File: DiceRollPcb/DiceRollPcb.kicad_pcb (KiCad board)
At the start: 2 copper layers, 96.5 x 68.6 mm, 20 parts, among them SW1 SW_Push, SW2 SW_Push, SW3 SW_Push, SW4 SW_Push, U1 RaspberryPiPico

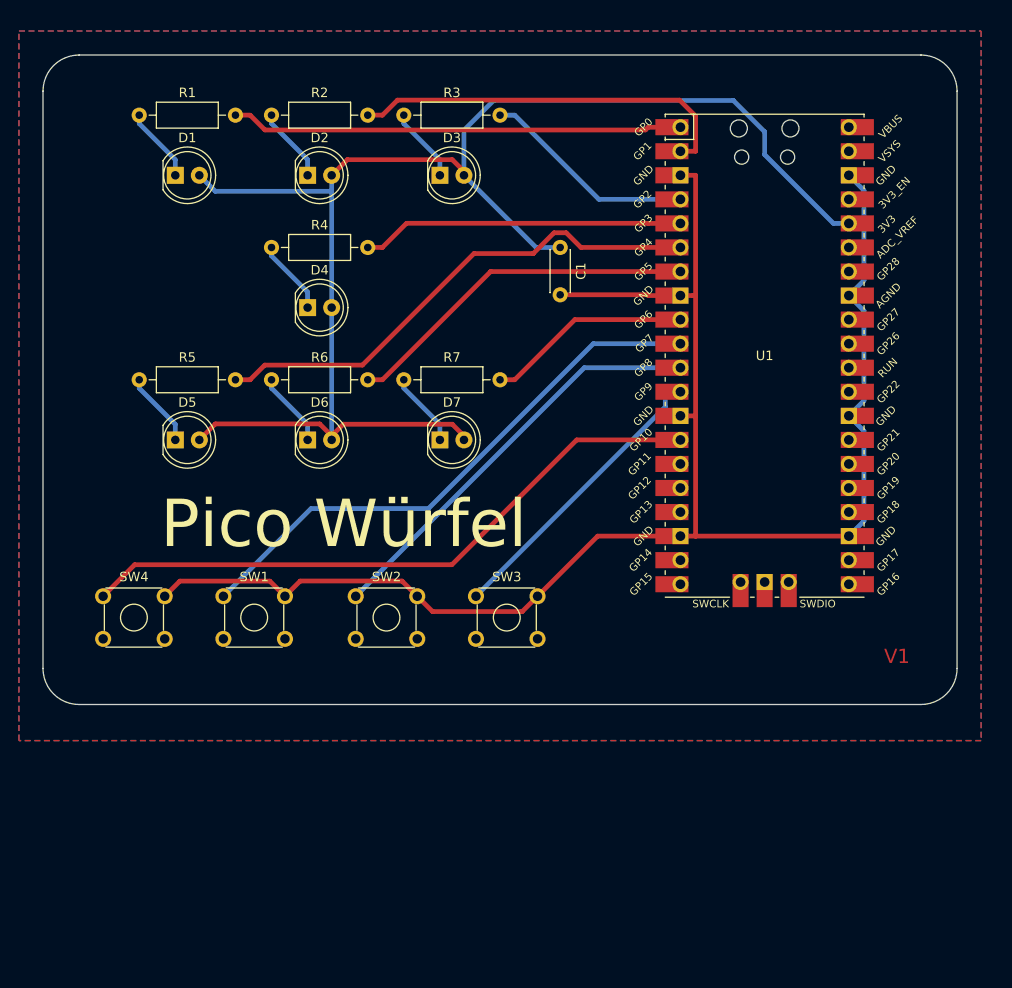
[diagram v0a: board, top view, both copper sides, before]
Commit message: Version 2
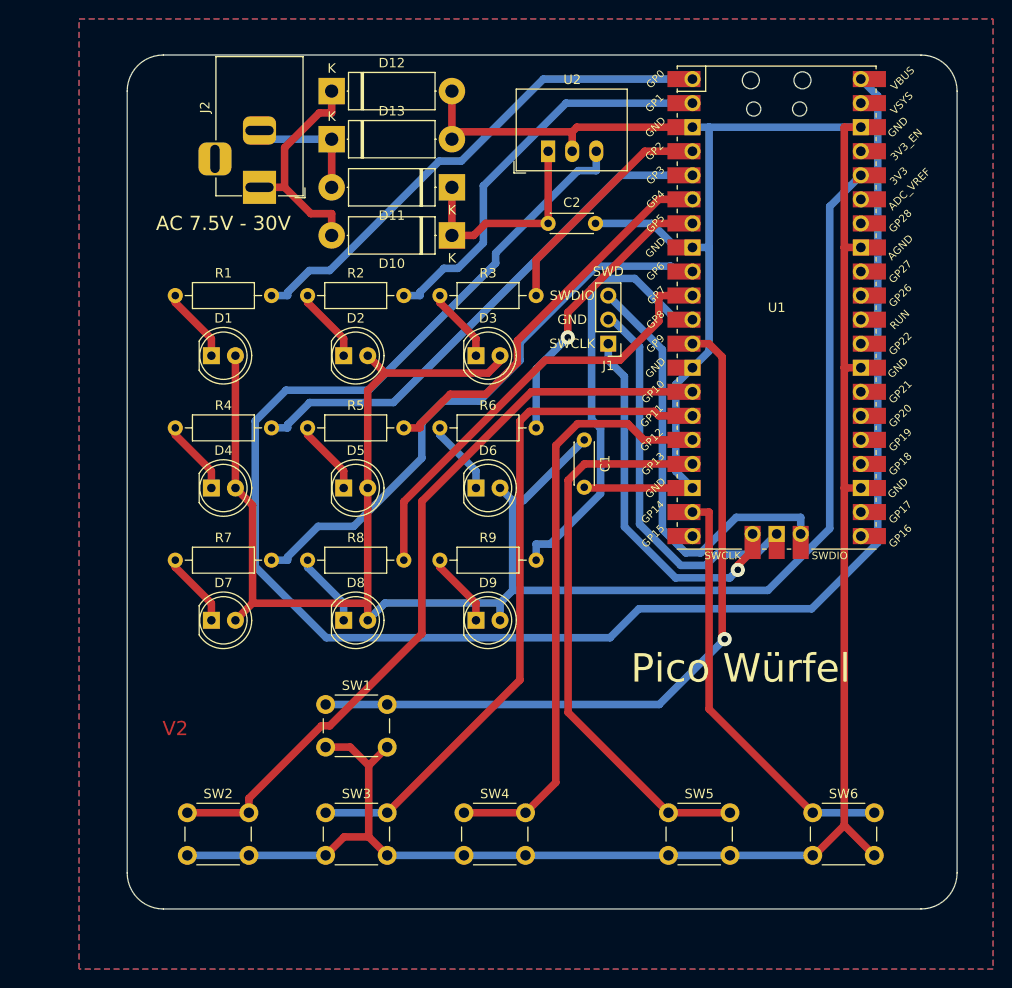
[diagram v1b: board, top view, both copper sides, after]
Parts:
- added C2: 4.7µF, Capacitor_THT:C_Disc_D4.3mm_W1.9mm_P5.00mm, F.Cu at (151.1, 74.9)
- added D10: D, Diode_THT:D_5W_P12.70mm_Horizontal, F.Cu at (141.0, 76.2)
- added D11: D, Diode_THT:D_5W_P12.70mm_Horizontal, F.Cu at (141.0, 71.1)
- added D12: D, Diode_THT:D_5W_P12.70mm_Horizontal, F.Cu at (128.3, 61.0)
- added D13: D, Diode_THT:D_5W_P12.70mm_Horizontal, F.Cu at (128.3, 66.0)
- added D8: LED, LED_THT:LED_D5.0mm, F.Cu at (129.5, 116.8)
- added D9: LED, LED_THT:LED_D5.0mm, F.Cu at (143.5, 116.8)
- added J1: Conn_01x03_Male, Connector_PinHeader_2.54mm:PinHeader_1x03_P2.54mm_Vertical, F.Cu at (157.5, 87.6)
- added J2: Barrel_Jack, Connector_BarrelJack:BarrelJack_Horizontal, F.Cu at (120.7, 71.1)
- added R8: R, Resistor_THT:R_Axial_DIN0207_L6.3mm_D2.5mm_P10.16mm_Horizontal, F.Cu at (125.7, 110.5)
- added R9: R, Resistor_THT:R_Axial_DIN0207_L6.3mm_D2.5mm_P10.16mm_Horizontal, F.Cu at (139.7, 110.5)
- added SW5: SW_Push, Button_Switch_THT:SW_PUSH_6mm, F.Cu at (163.8, 137.2)
- added SW6: SW_Push, Button_Switch_THT:SW_PUSH_6mm, F.Cu at (179.1, 137.2)
- added U2: R-785.0-0.5, Converter_DCDC:Converter_DCDC_RECOM_R-78E-0.5_THT, F.Cu at (151.1, 67.3)
- SW1, SW2, SW3, SW4: footprint Button_Switch_THT:SW_TH_Tactile_Omron_B3F-10xx -> Button_Switch_THT:SW_PUSH_6mm
- moved SW4 44.4 mm to (142.2, 137.2)
- moved D7 30.7 mm to (115.6, 116.8)
- moved R7 30.7 mm to (111.8, 110.5)
- moved SW2 29.0 mm to (113.0, 137.2)
- moved SW3 27.8 mm to (127.6, 137.2)
- moved D4 21.6 mm to (115.6, 102.9)
- moved R4 21.6 mm to (111.8, 96.5)
- moved C1 20.5 mm to (154.9, 97.8)
- moved D3 19.4 mm to (143.5, 88.9)
- moved D1 19.4 mm to (115.6, 88.9)
- moved D2 19.4 mm to (129.5, 88.9)
- moved R1 19.4 mm to (111.8, 82.5)
- moved R2 19.4 mm to (125.7, 82.5)
- moved R3 19.4 mm to (139.7, 82.5)
- moved R5 18.5 mm to (125.7, 96.5)
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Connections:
- U1 pad 10: SWITCH1 -> LED8
- U1 pad 11: SWITCH2 -> LED9
- U1 pad 12: SWITCH3 -> SWITCH1
- U1 pad 14: SWITCH4 -> SWITCH2
- U1 pad 15: Net-(U1-Pad15) -> SWITCH3
- U1 pad 16: Net-(U1-Pad16) -> SWITCH4
- U1 pad 17: Net-(U1-Pad17) -> SWITCH5
- U1 pad 19: Net-(U1-Pad19) -> SWITCH6
- U1 pad 40: Net-(U1-Pad40) -> +5V
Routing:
- net +5V: track 0.00 -> 187.7 mm
- net GND: track 176.6 -> 288.4 mm
- net SWITCH5: track 0.00 -> 59.8 mm
- net LED8: track 0.00 -> 47.3 mm
- net Net-(J1-Pad3): track 0.00 -> 46.0 mm
- net LED9: track 0.00 -> 45.7 mm
- net SWITCH6: track 0.00 -> 44.5 mm
- net +3V3: track 156.0 -> 199.1 mm
- net SWITCH3: track 31.5 -> 72.5 mm
- net Net-(J1-Pad2): track 0.00 -> 40.9 mm
- net LED7: track 21.7 -> 61.0 mm
- net Net-(J1-Pad1): track 0.00 -> 39.0 mm, vias 0 -> 1
- net SWITCH2: track 44.3 -> 80.8 mm
- net /AC_1: track 0.00 -> 24.0 mm
- net /DC_PLUS: track 0.00 -> 23.9 mm
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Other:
- board size 96.5 x 68.6 mm -> 87.6 x 90.2 mm
- net class Default: trace_width 0.5 -> 0.8; via_dia 1 -> 1.5; via_drill 0.5 -> 0.7
- net class Power added: clearance 0.5, trace_width 0.8, via_dia 1.5, via_drill 0.7
- board text added: "AC 7.5V - 30V"
- board text added: "GND"
- board text added: "SWCLK"
- board text added: "SWD"
- board text added: "SWDIO"
- board text added: "V2"
- board text removed: "V1"
